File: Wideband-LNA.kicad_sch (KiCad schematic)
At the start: 25 parts, among them J1 RF-IN, J2 RF-OUT, J3 USB_C_Receptacle_USB2.0_16P, U1 TQP3M9036, U2 AP2127K-ADJ

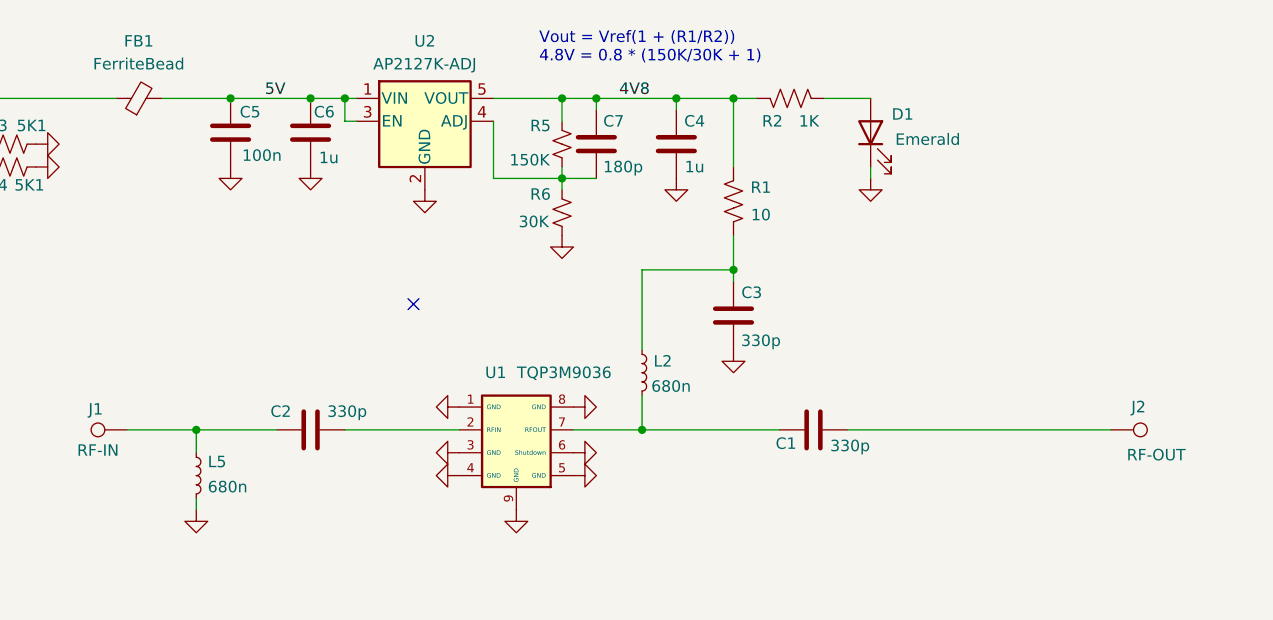
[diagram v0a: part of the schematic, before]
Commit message: Preparing for fab and assy
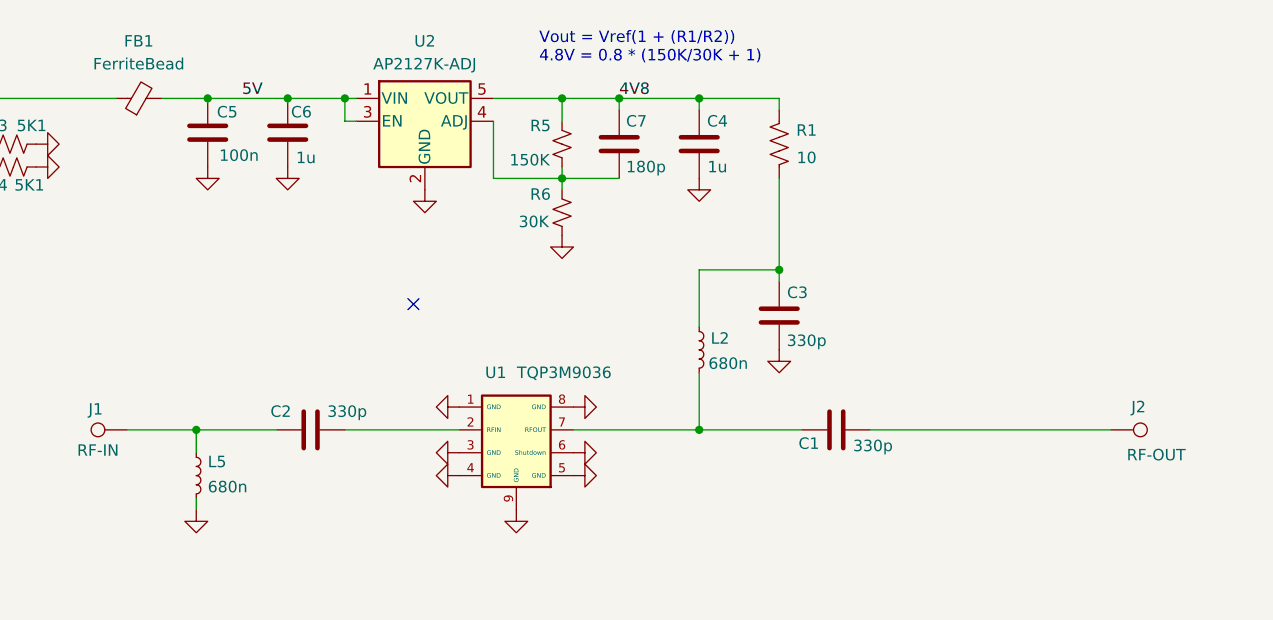
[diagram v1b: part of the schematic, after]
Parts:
- removed D1: Emerald, Diode_SMD:D_0402_1005Metric, symbol Device:LED
- removed R2: 1K, Resistor_SMD:R_0402_1005Metric, symbol Device:R_US
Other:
- moved on the sheet: C1, C3, C4, C5, C6, C7, L2, R1
